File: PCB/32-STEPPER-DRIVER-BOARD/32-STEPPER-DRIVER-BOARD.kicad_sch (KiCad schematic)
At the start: 346 parts, among them J1 MEC2-30-01-X-TH1-NP-WT, J2 MEC2-30-01-X-TH1-NP-WT, J3 MEC2-30-01-X-TH1-NP-WT, J4 MEC2-30-01-X-TH1-NP-WT, U1 74HC595, U10 74HC595, U11 74HC595, U12 74HC595, U13 74HC595, U14 74HC595, U15 74HC595, U17 74HC595, U18 74HC595, U19 74HC595, U2 74HC595, U20 74HC595, U21 74HC595, U22 74HC595, U3 74HC595, U4 74HC595, U5 74HC595, U6 74HC595, U7 74HC595, U9 74HC595

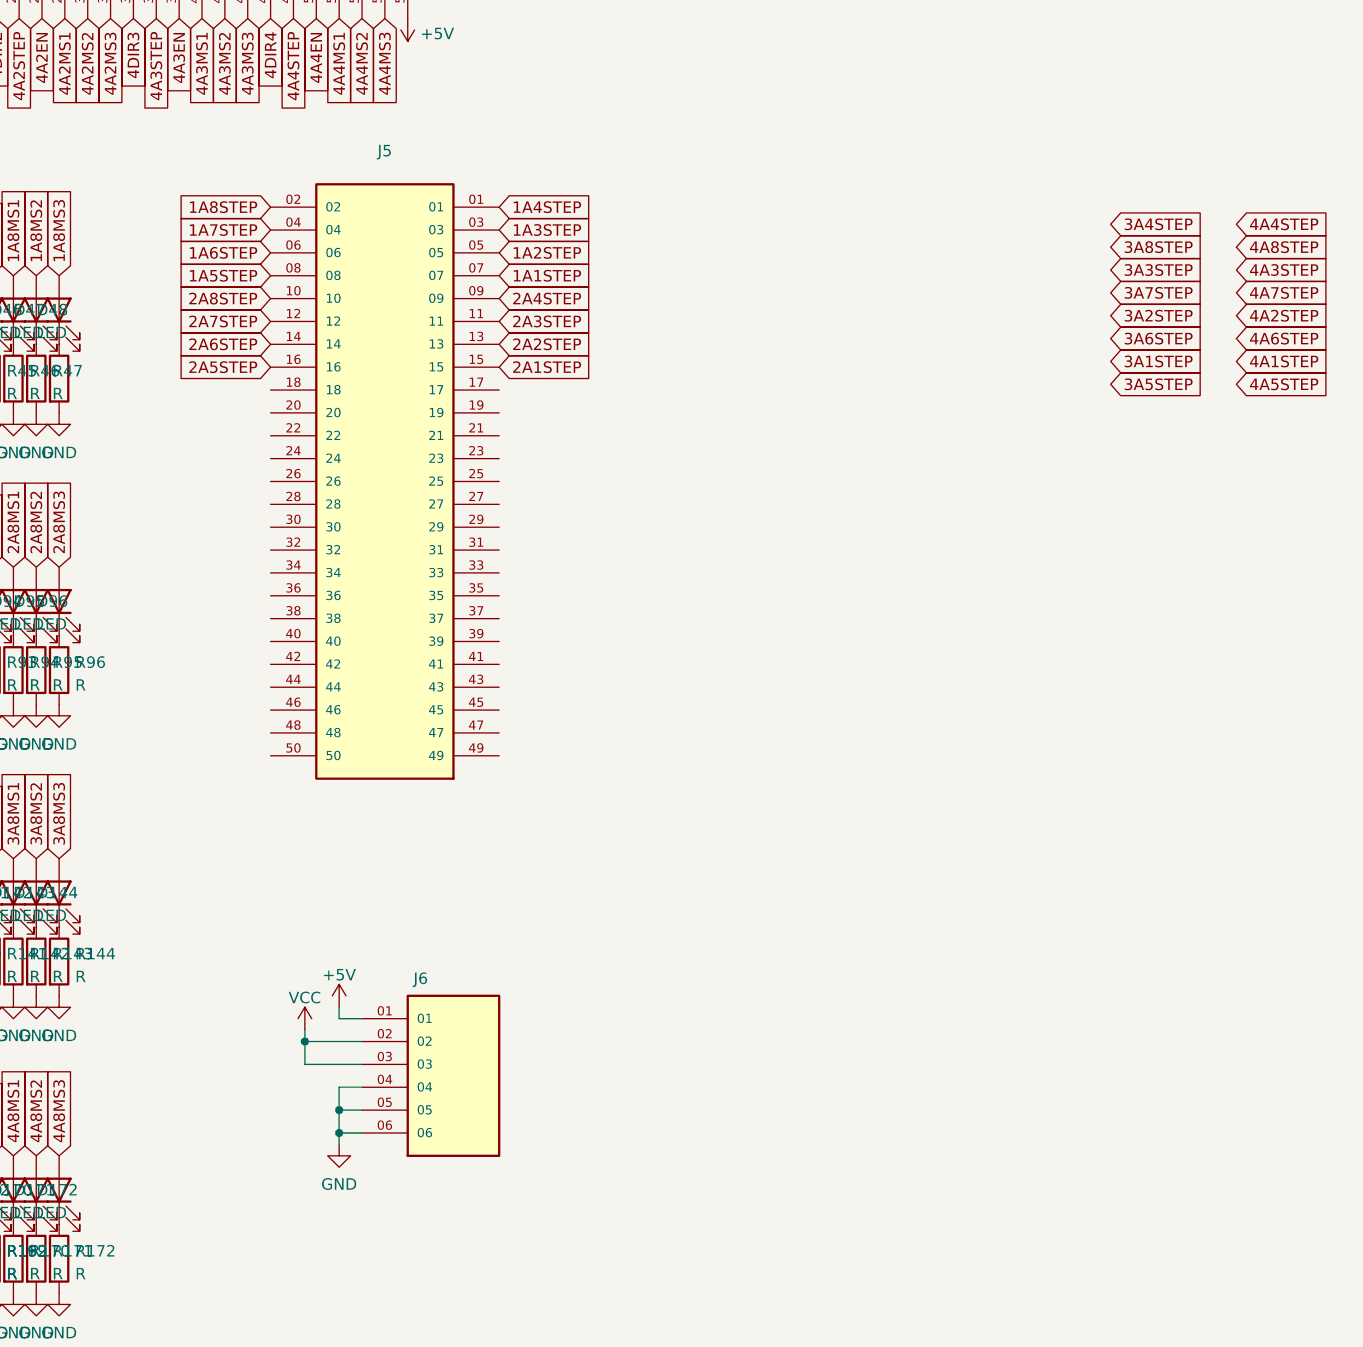
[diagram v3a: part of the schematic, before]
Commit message: progress
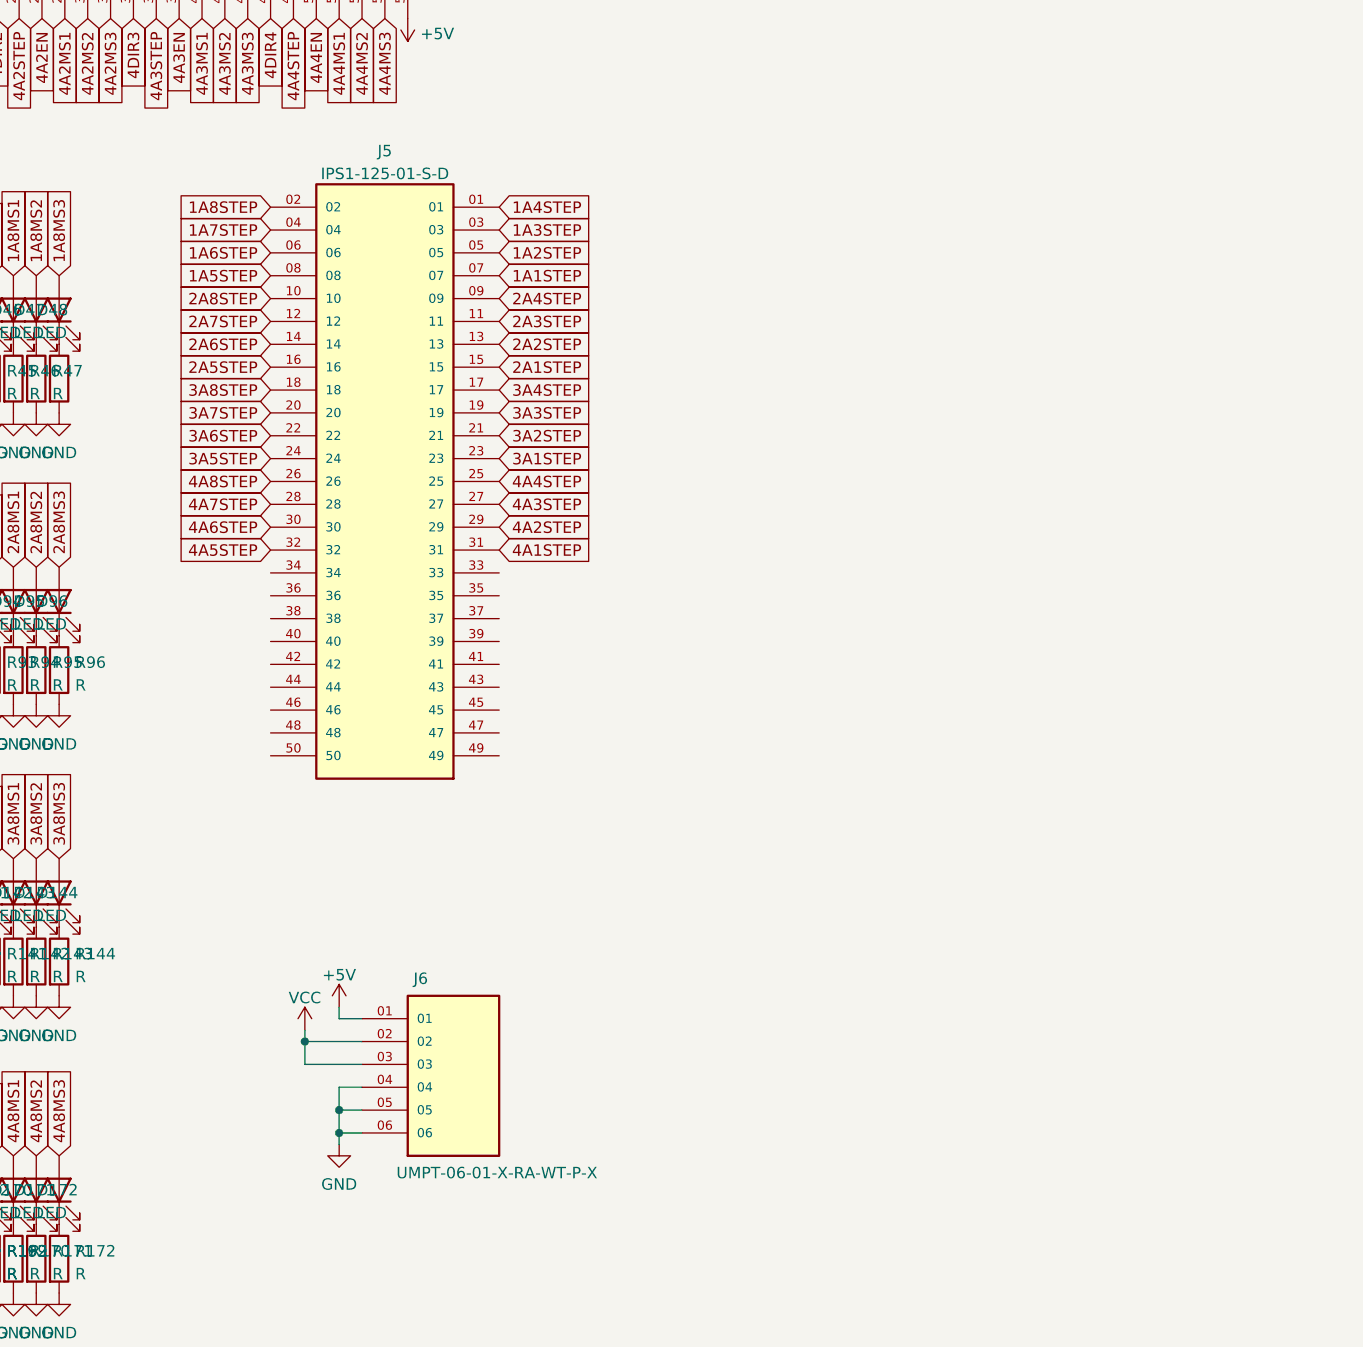
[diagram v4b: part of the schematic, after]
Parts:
- J5: value (none) -> IPS1-125-01-S-D; footprint (none) -> LIBRARIES:SAMTEC_IPS1-125-01-S-D
- J6: value (none) -> UMPT-06-01-X-RA-WT-P-X; footprint (none) -> LIBRARIES:SAMTEC_UMPT-06-01-X-RA-WT-P-X
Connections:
- net 3A1STEP: now also J5.23
- net 3A2STEP: now also J5.21
- net 3A3STEP: now also J5.19
- net 3A4STEP: now also J5.17
- net 3A5STEP: now also J5.24
- net 3A6STEP: now also J5.22
- net 3A7STEP: now also J5.20
- net 3A8STEP: now also J5.18
- net 4A1STEP: now also J5.31
- net 4A2STEP: now also J5.29
- net 4A3STEP: now also J5.27
- net 4A4STEP: now also J5.25
- net 4A5STEP: now also J5.32
- net 4A6STEP: now also J5.30
- net 4A7STEP: now also J5.28
- net 4A8STEP: now also J5.26
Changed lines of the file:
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@@
     )
   )
-  (global_label "3A6STEP" (shape input) (at 467.36 86.36 0) (fields_autoplaced)
-    (effects (font (size 1.27 1.27)) (justify left))
-    (property "Intersheet References" "${INTERSHEET_REFS}" (id 0) (at 477.8769 86.2806 0)
-      (effects (font (size 1.27 1.27)) (justify left) hide)
+  (global_label "3A6STEP" (shape input) (at 374.015 97.155 180) (fields_autoplaced)
+    (effects (font (size 1.27 1.27)) (justify right))
+    (property "Intersheet References" "${INTERSHEET_REFS}" (id 0) (at 363.4981 97.2344 0)
+      (effects (font (size 1.27 1.27)) (justify right) hide)
     )
   )
@@
     )
   )
-  (global_label "3A3STEP" (shape input) (at 467.36 78.74 0) (fields_autoplaced)
+  (global_label "3A3STEP" (shape input) (at 399.415 94.615 0) (fields_autoplaced)
     (effects (font (size 1.27 1.27)) (justify left))
-    (property "Intersheet References" "${INTERSHEET_REFS}" (id 0) (at 477.8769 78.6606 0)
+    (property "Intersheet References" "${INTERSHEET_REFS}" (id 0) (at 409.9319 94.5356 0)
       (effects (font (size 1.27 1.27)) (justify left) hide)
     )
@@
     )
   )
-  (global_label "4A6STEP" (shape input) (at 481.33 86.36 0) (fields_autoplaced)
-    (effects (font (size 1.27 1.27)) (justify left))
-    (property "Intersheet References" "${INTERSHEET_REFS}" (id 0) (at 491.8469 86.2806 0)
-      (effects (font (size 1.27 1.27)) (justify left) hide)
+  (global_label "4A6STEP" (shape input) (at 374.015 107.315 180) (fields_autoplaced)
+    (effects (font (size 1.27 1.27)) (justify right))
+    (property "Intersheet References" "${INTERSHEET_REFS}" (id 0) (at 363.4981 107.3944 0)
+      (effects (font (size 1.27 1.27)) (justify right) hide)
     )
   )
@@
     )
   )
-  (global_label "4A2STEP" (shape input) (at 481.33 83.82 0) (fields_autoplaced)
+  (global_label "4A2STEP" (shape input) (at 399.415 107.315 0) (fields_autoplaced)
     (effects (font (size 1.27 1.27)) (justify left))
-    (property "Intersheet References" "${INTERSHEET_REFS}" (id 0) (at 491.8469 83.7406 0)
+    (property "Intersheet References" "${INTERSHEET_REFS}" (id 0) (at 409.9319 107.2356 0)
       (effects (font (size 1.27 1.27)) (justify left) hide)
     )
@@
     )
   )
-  (global_label "4A8STEP" (shape input) (at 481.33 76.2 0) (fields_autoplaced)
-    (effects (font (size 1.27 1.27)) (justify left))
-    (property "Intersheet References" "${INTERSHEET_REFS}" (id 0) (at 491.8469 76.1206 0)
-      (effects (font (size 1.27 1.27)) (justify left) hide)
+  (global_label "4A8STEP" (shape input) (at 374.015 102.235 180) (fields_autoplaced)
+    (effects (font (size 1.27 1.27)) (justify right))
+    (property "Intersheet References" "${INTERSHEET_REFS}" (id 0) (at 363.4981 102.3144 0)
+      (effects (font (size 1.27 1.27)) (justify right) hide)
     )
   )
@@
     )
   )
-  (global_label "4A7STEP" (shape input) (at 481.33 81.28 0) (fields_autoplaced)
-    (effects (font (size 1.27 1.27)) (justify left))
-    (property "Intersheet References" "${INTERSHEET_REFS}" (id 0) (at 491.8469 81.2006 0)
-      (effects (font (size 1.27 1.27)) (justify left) hide)
+  (global_label "4A7STEP" (shape input) (at 374.015 104.775 180) (fields_autoplaced)
+    (effects (font (size 1.27 1.27)) (justify right))
+    (property "Intersheet References" "${INTERSHEET_REFS}" (id 0) (at 363.4981 104.8544 0)
+      (effects (font (size 1.27 1.27)) (justify right) hide)
     )
   )
@@
     )
   )
-  (global_label "3A7STEP" (shape input) (at 467.36 81.28 0) (fields_autoplaced)
-    (effects (font (size 1.27 1.27)) (justify left))
-    (property "Intersheet References" "${INTERSHEET_REFS}" (id 0) (at 477.8769 81.2006 0)
-      (effects (font (size 1.27 1.27)) (justify left) hide)
+  (global_label "3A7STEP" (shape input) (at 374.015 94.615 180) (fields_autoplaced)
+    (effects (font (size 1.27 1.27)) (justify right))
+    (property "Intersheet References" "${INTERSHEET_REFS}" (id 0) (at 363.4981 94.6944 0)
+      (effects (font (size 1.27 1.27)) (justify right) hide)
     )
   )
@@
     )
   )
-  (global_label "4A1STEP" (shape input) (at 481.33 88.9 0) (fields_autoplaced)
+  (global_label "4A1STEP" (shape input) (at 399.415 109.855 0) (fields_autoplaced)
     (effects (font (size 1.27 1.27)) (justify left))
-    (property "Intersheet References" "${INTERSHEET_REFS}" (id 0) (at 491.8469 88.8206 0)
+    (property "Intersheet References" "${INTERSHEET_REFS}" (id 0) (at 409.9319 109.7756 0)
       (effects (font (size 1.27 1.27)) (justify left) hide)
     )
@@
     )
   )
-  (global_label "4A5STEP" (shape input) (at 481.33 91.44 0) (fields_autoplaced)
-    (effects (font (size 1.27 1.27)) (justify left))
-    (property "Intersheet References" "${INTERSHEET_REFS}" (id 0) (at 491.8469 91.3606 0)
-      (effects (font (size 1.27 1.27)) (justify left) hide)
+  (global_label "4A5STEP" (shape input) (at 374.015 109.855 180) (fields_autoplaced)
+    (effects (font (size 1.27 1.27)) (justify right))
+    (property "Intersheet References" "${INTERSHEET_REFS}" (id 0) (at 363.4981 109.9344 0)
+      (effects (font (size 1.27 1.27)) (justify right) hide)
     )
   )
@@
     )
   )
-  (global_label "3A4STEP" (shape input) (at 467.36 73.66 0) (fields_autoplaced)
+  (global_label "3A4STEP" (shape input) (at 399.415 92.075 0) (fields_autoplaced)
     (effects (font (size 1.27 1.27)) (justify left))
-    (property "Intersheet References" "${INTERSHEET_REFS}" (id 0) (at 477.8769 73.5806 0)
+    (property "Intersheet References" "${INTERSHEET_REFS}" (id 0) (at 409.9319 91.9956 0)
       (effects (font (size 1.27 1.27)) (justify left) hide)
     )
@@
     )
   )
-  (global_label "3A1STEP" (shape input) (at 467.36 88.9 0) (fields_autoplaced)
+  (global_label "3A1STEP" (shape input) (at 399.415 99.695 0) (fields_autoplaced)
     (effects (font (size 1.27 1.27)) (justify left))
-    (property "Intersheet References" "${INTERSHEET_REFS}" (id 0) (at 477.8769 88.8206 0)
+    (property "Intersheet References" "${INTERSHEET_REFS}" (id 0) (at 409.9319 99.6156 0)
       (effects (font (size 1.27 1.27)) (justify left) hide)
     )
@@
     )
   )
-  (global_label "3A2STEP" (shape input) (at 467.36 83.82 0) (fields_autoplaced)
+  (global_label "3A2STEP" (shape input) (at 399.415 97.155 0) (fields_autoplaced)
     (effects (font (size 1.27 1.27)) (justify left))
-    (property "Intersheet References" "${INTERSHEET_REFS}" (id 0) (at 477.8769 83.7406 0)
+    (property "Intersheet References" "${INTERSHEET_REFS}" (id 0) (at 409.9319 97.0756 0)
       (effects (font (size 1.27 1.27)) (justify left) hide)
     )
@@
     )
   )
-  (global_label "3A5STEP" (shape input) (at 467.36 91.44 0) (fields_autoplaced)
-    (effects (font (size 1.27 1.27)) (justify left))
-    (property "Intersheet References" "${INTERSHEET_REFS}" (id 0) (at 477.8769 91.3606 0)
-      (effects (font (size 1.27 1.27)) (justify left) hide)
+  (global_label "3A5STEP" (shape input) (at 374.015 99.695 180) (fields_autoplaced)
+    (effects (font (size 1.27 1.27)) (justify right))
+    (property "Intersheet References" "${INTERSHEET_REFS}" (id 0) (at 363.4981 99.7744 0)
+      (effects (font (size 1.27 1.27)) (justify right) hide)
     )
   )
@@
     )
   )
-  (global_label "4A3STEP" (shape input) (at 481.33 78.74 0) (fields_autoplaced)
+  (global_label "4A3STEP" (shape input) (at 399.415 104.775 0) (fields_autoplaced)
     (effects (font (size 1.27 1.27)) (justify left))
-    (property "Intersheet References" "${INTERSHEET_REFS}" (id 0) (at 491.8469 78.6606 0)
+    (property "Intersheet References" "${INTERSHEET_REFS}" (id 0) (at 409.9319 104.6956 0)
       (effects (font (size 1.27 1.27)) (justify left) hide)
     )
@@
     )
   )
-  (global_label "4A4STEP" (shape input) (at 481.33 73.66 0) (fields_autoplaced)
+  (global_label "4A4STEP" (shape input) (at 399.415 102.235 0) (fields_autoplaced)
     (effects (font (size 1.27 1.27)) (justify left))
-    (property "Intersheet References" "${INTERSHEET_REFS}" (id 0) (at 491.8469 73.5806 0)
+    (property "Intersheet References" "${INTERSHEET_REFS}" (id 0) (at 409.9319 102.1556 0)
       (effects (font (size 1.27 1.27)) (justify left) hide)
     )
@@
     )
   )
-  (global_label "3A8STEP" (shape input) (at 467.36 76.2 0) (fields_autoplaced)
-    (effects (font (size 1.27 1.27)) (justify left))
-    (property "Intersheet References" "${INTERSHEET_REFS}" (id 0) (at 477.8769 76.1206 0)
-      (effects (font (size 1.27 1.27)) (justify left) hide)
+  (global_label "3A8STEP" (shape input) (at 374.015 92.075 180) (fields_autoplaced)
+    (effects (font (size 1.27 1.27)) (justify right))
+    (property "Intersheet References" "${INTERSHEET_REFS}" (id 0) (at 363.4981 92.1544 0)
+      (effects (font (size 1.27 1.27)) (justify right) hide)
     )
   )
@@
       (effects (font (size 1.27 1.27)) (justify left))
     )
-    (property "Value" "" (id 1) (at 387.985 179.07 0)
+    (property "Value" "UMPT-06-01-X-RA-WT-P-X" (id 1) (at 387.985 179.07 0)
       (effects (font (size 1.27 1.27)) (justify left))
     )
-    (property "Footprint" "" (id 2) (at 394.335 167.005 0)
+    (property "Footprint" "LIBRARIES:SAMTEC_UMPT-06-01-X-RA-WT-P-X" (id 2) (at 394.335 167.005 0)
       (effects (font (size 1.27 1.27)) (justify left bottom) hide)
     )
@@
     (in_bom yes) (on_board yes) (fields_autoplaced)
     (property "Reference" "J5" (id 0) (at 386.715 65.5152 0))
-    (property "Value" "" (id 1) (at 386.715 68.0521 0))
-    (property "Footprint" "" (id 2) (at 386.715 102.235 0)
+    (property "Value" "IPS1-125-01-S-D" (id 1) (at 386.715 68.0521 0))
+    (property "Footprint" "LIBRARIES:SAMTEC_IPS1-125-01-S-D" (id 2) (at 386.715 102.235 0)
       (effects (font (size 1.27 1.27)) (justify left bottom) hide)
     )
